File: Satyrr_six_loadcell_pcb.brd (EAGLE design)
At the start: 36 x 76 mm, 49 parts, among them IC1 STM32G431KBU6, J2 SM02BGHSTBLFSN, J3 SM04B-GHS-TB(LF)(SN)-, J4 SM04B-GHS-TB(LF)(SN)-, J5 SM04B-GHS-TB(LF)(SN)-, J6 SM04B-GHS-TB(LF)(SN)-, J7 SM04B-GHS-TB(LF)(SN)-, J8 SM04B-GHS-TB(LF)(SN)-, J9 22057025, U1 MCP2562FD-H/MFDFN8_3X3MC_MCH-M, U2 AP7361C-33Y5-13SOT89-5_DIO-M, Y1 ECS-80-18-33-JGN-TR

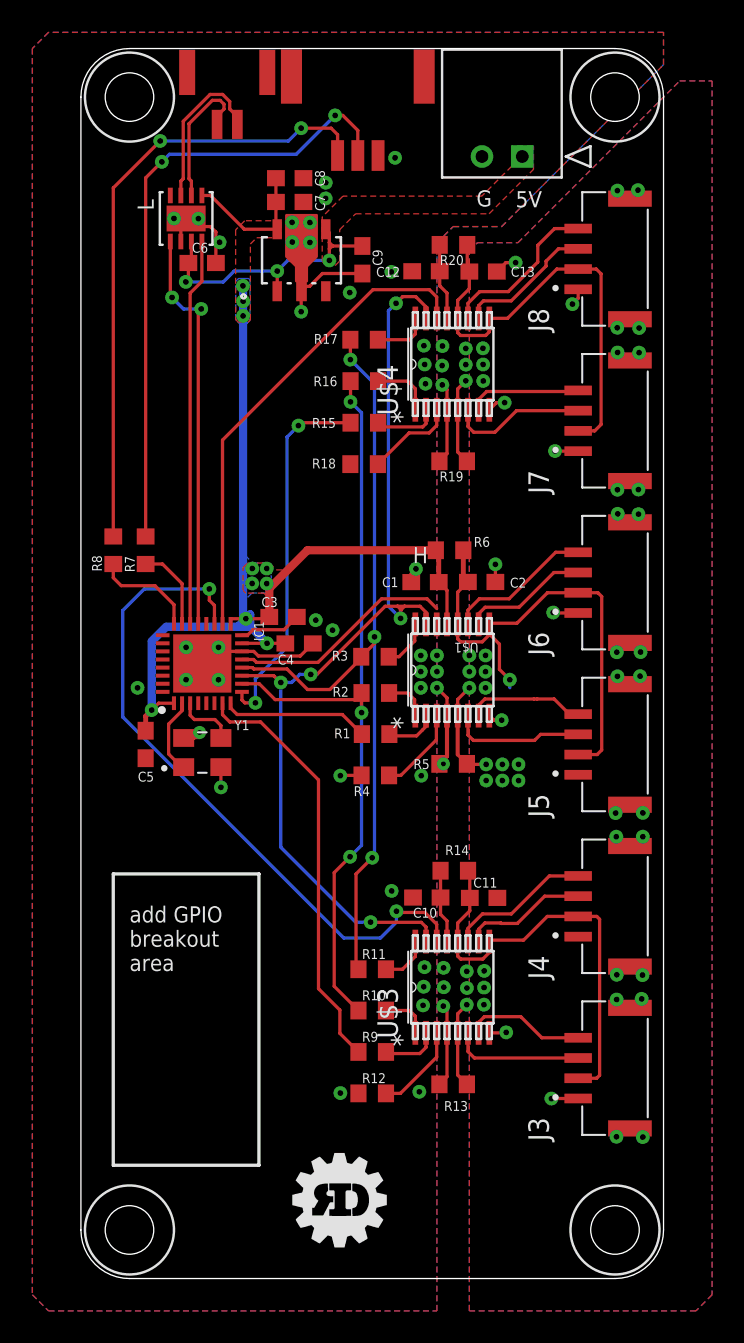
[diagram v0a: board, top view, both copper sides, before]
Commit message: board finished, ready for design review
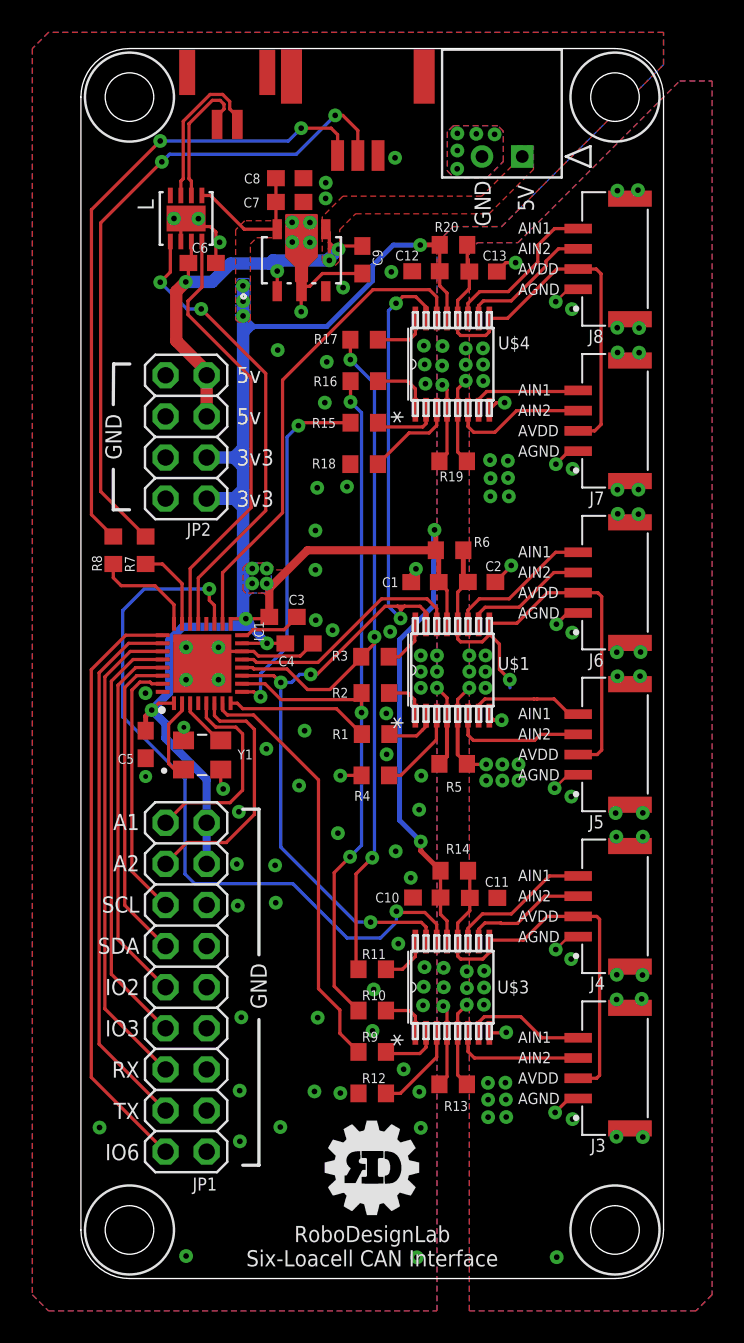
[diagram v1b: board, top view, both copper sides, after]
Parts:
- added JP1: (no value), pinhead:2X09
- added JP2: (no value), pinhead:2X04
- moved Y1 0.15 mm to (7.49, 32.4)
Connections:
- removed net N$13: IC1.5
- removed net N$14: IC1.6
- removed net N$34: IC1.31
- removed net N$35: IC1.30
- removed net N$36: IC1.29
- removed net N$37: IC1.28
- removed net N$38: IC1.27
- removed net N$39: IC1.26
- removed net N$40: IC1.25
- new net GPIO0_SCL: IC1.31, JP1.5
- new net GPIO1_SDA: IC1.30, JP1.7
- new net GPIO2: IC1.29, JP1.9
- new net GPIO3: IC1.28, JP1.11
- new net GPIO4_RX: IC1.27, JP1.13
- new net GPIO5_TX: IC1.26, JP1.15
- new net GPIO6: IC1.25, JP1.17
- new net GPIO7_ADC1: IC1.5, JP1.1
- new net GPIO8_ADC2: IC1.6, JP1.3
- net 3V3: now also JP1.2, JP1.4, JP2.1, JP2.3
- net 5V: now also JP2.5, JP2.7
- net GND: now also JP1.10, JP1.12, JP1.14, JP1.16, JP1.18, JP1.6, JP1.8, JP2.2, JP2.4, JP2.6, JP2.8
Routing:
- net 3V3: track 79.0 -> 138.1 mm, vias 10 -> 13
- net GPIO6: track 0.00 -> 37.0 mm
- net GPIO5_TX: track 0.00 -> 33.4 mm
- net GPIO4_RX: track 0.00 -> 30.0 mm
- net GPIO3: track 0.00 -> 26.6 mm
- net GPIO2: track 0.00 -> 23.1 mm
- net GPIO1_SDA: track 0.00 -> 19.7 mm
- net GPIO0_SCL: track 0.00 -> 16.3 mm
- net GPIO8_ADC2: track 0.00 -> 15.6 mm
- net GPIO7_ADC1: track 0.00 -> 12.6 mm
- net 5V: track 17.7 -> 28.8 mm, vias 3 -> 4
- net AGND: track 29.1 -> 33.5 mm, vias 57 -> 78
- net FDCAN_RX: track 25.1 -> 28.8 mm
- net DRDY_2: track 42.3 -> 45.8 mm
- net FDCAN_TX: track 23.9 -> 27.2 mm
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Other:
- board text added: "1"
- board text added: "2"
- board text added: "3"
- board text added: "4"
- board text added: "5"
- board text added: "5v 5v 3v3 3v3"
- board text added: "6"
- board text added: "A1 A2 SCL SDA IO2 IO3 RX TX IO6"
- board text added: "GND"
- board text added: "LoadCells"
- board text added: "RoboDesignLab Six-Loacell CAN Interface"
- board text removed: "G"
- board text removed: "H"
- board text removed: "Six-Loadcell CAN Interface PCB"
- board text removed: "add GPIO breakout area"
